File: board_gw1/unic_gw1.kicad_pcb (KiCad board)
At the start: 4 copper layers, 49.5 x 15.2 mm, 112 parts, among them Q1 2N7002, Q10 2N7002, Q11 2N7002, Q12 2N7002, Q13 2N7002, Q14 2N7002, Q15 2N7002, Q16 2N7002, Q17 2N7002, Q18 2N7002, Q19 2N7002, Q2 2N7002, Q20 2N7002, Q21 2N7002, Q22 2N7002, Q23 2N7002, Q24 2N7002, Q25 2N7002, Q26 2N7002, Q27 2N7002, Q28 2N7002, Q29 2N7002, Q3 2N7002, Q30 2N7002, Q31 2N7002, Q32 2N7002, Q33 2N7002, Q34 2N7002, Q35 2N7002, Q36 2N7002, Q37 2N7002, Q38 2N7002, Q39 2N7002, Q4 2N7002, Q40 2N7002, Q5 2N7002, Q6 2N7002, Q7 2N7002, Q8 2N7002, Q9 2N7002, U1 GW1N-LV9QN88C6_I5_, U2 LM3480-3.3, U3 AP2202K-ADJ, U4 ESP-PSRAM32, U5 AT25SF081-XMHF-X, U6 AP62150Z6, X1 ASE-xxxMHz

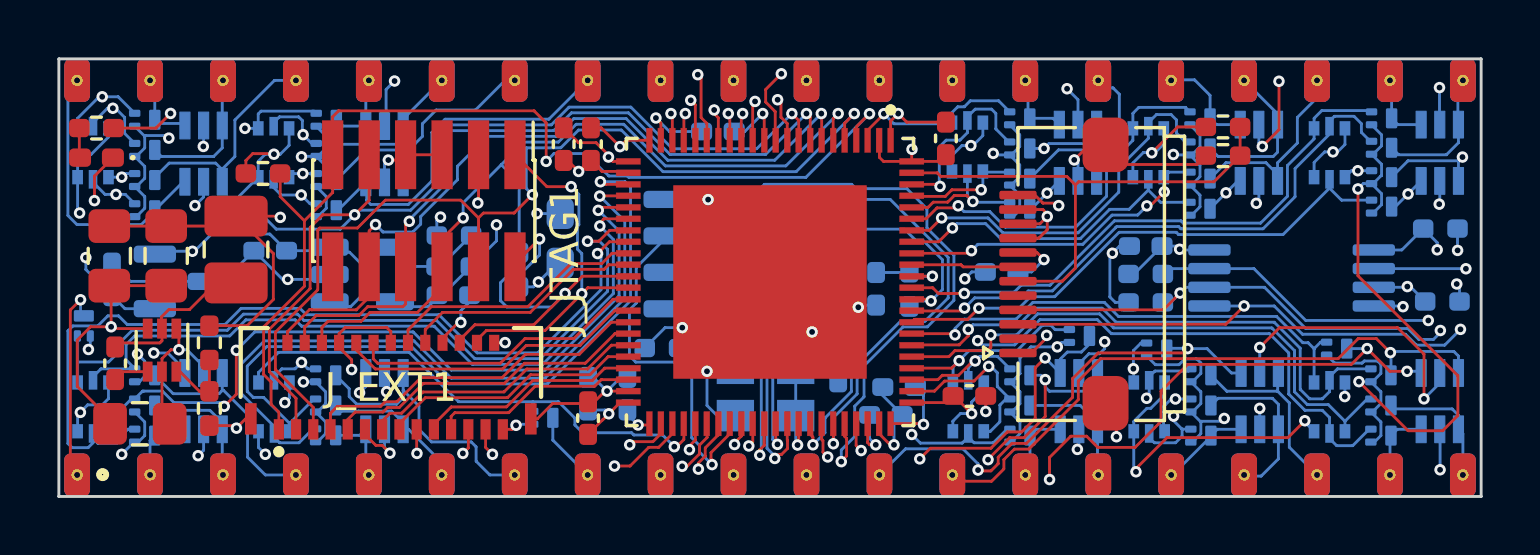
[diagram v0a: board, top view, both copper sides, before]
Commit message: Board more or less done.
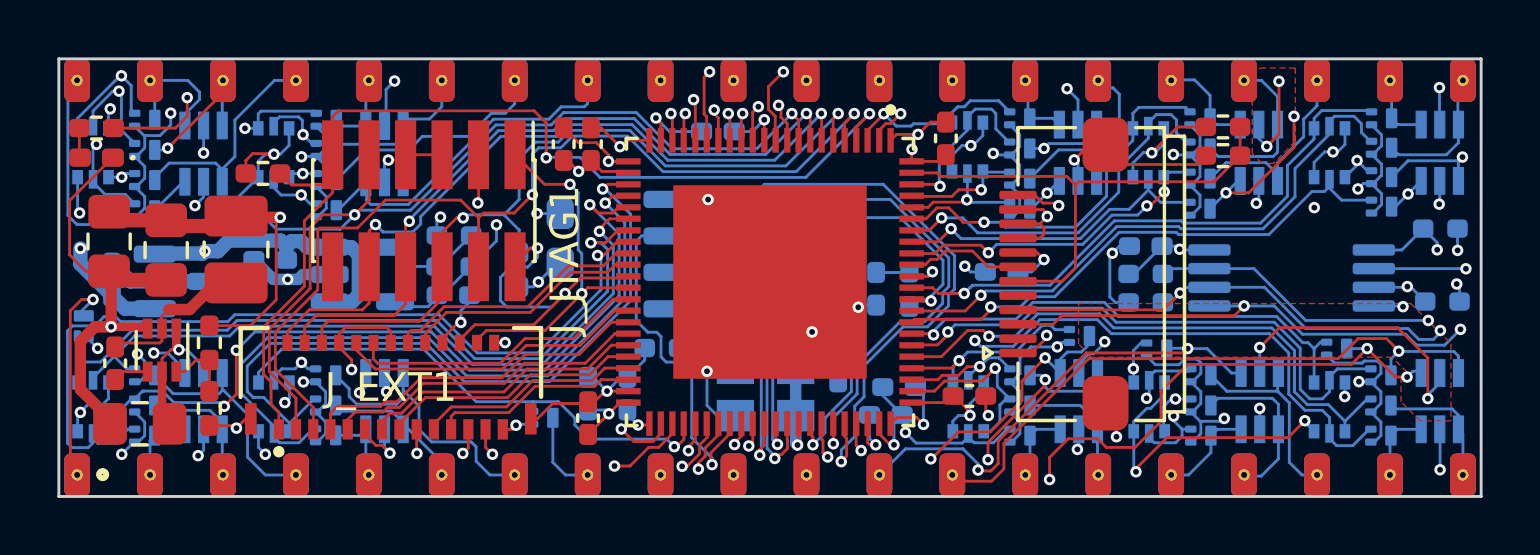
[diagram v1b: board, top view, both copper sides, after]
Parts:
- moved C7 0.50 mm to (126.2, 94.0)
- moved C1 0.32 mm to (131.8, 94.6)
- moved C8 0.20 mm to (128.2, 94.3)
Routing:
- net +5V: track 186.6 -> 149.4 mm, vias 14 -> 15
- net GND: track 223.1 -> 215.5 mm, vias 38 -> 37
- net /PIN29: track 15.1 -> 20.4 mm, vias 1 -> 2
- net /PIN39: track 2.05 -> 4.47 mm
- net /PIN30: track 24.3 -> 25.7 mm
- net /PIN38_F: track 24.5 -> 25.7 mm
- net +3V3: track 222.4 -> 223.6 mm, vias 28 -> 29
- net /JTAG_TDO: track 25.9 -> 24.8 mm
- net /RECONFIG_N: track 35.9 -> 34.7 mm
- net /JTAG_TCK: track 26.7 -> 25.7 mm
- net /PIN8: track 12.4 -> 13.5 mm
- net /PIN6_F: track 25.8 -> 25.0 mm
- net /JTAG_SEL_N: track 36.9 -> 37.6 mm
- net /PIN3_F: track 26.7 -> 27.4 mm
- net /PIN34: track 8.45 -> 9.15 mm
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- added copper zone on In2.Cu, net +1V2
- added copper zone on In1.Cu, net +3V3
- added copper zone on In2.Cu, net +3V3
- added copper zone on In1.Cu, net +5V
- added copper zone on In2.Cu, net +5V
- added copper zone on In1.Cu, net GND
- added copper zone on F.Cu, net LINE
- added copper zone on In1.Cu, net LINE
- added copper zone on In2.Cu, net LINE
